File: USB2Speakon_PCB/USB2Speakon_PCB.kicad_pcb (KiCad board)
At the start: 4 copper layers, 15 x 26 mm, 51 parts, among them J1 USB_C_Receptacle_USB2.0_16P, J2 Conn_01x04, U1 PCM2912A, U2 TPA2012D2RTJR, Y1 6 MHz

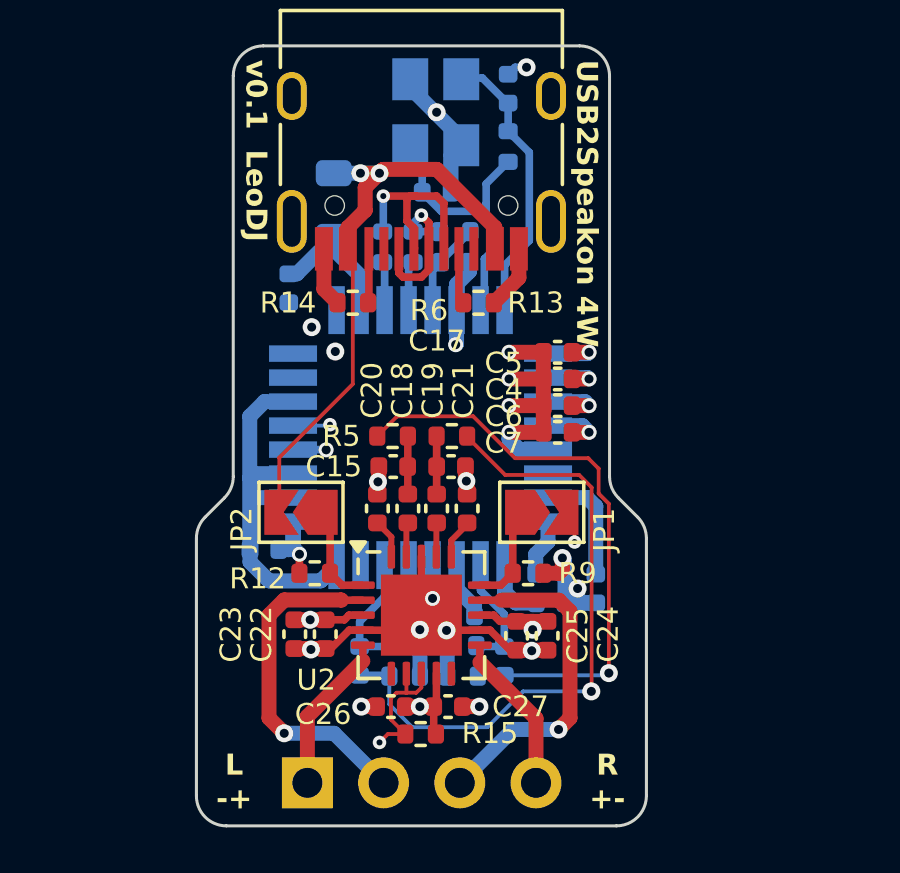
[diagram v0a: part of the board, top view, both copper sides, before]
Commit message: some minor changes, idk
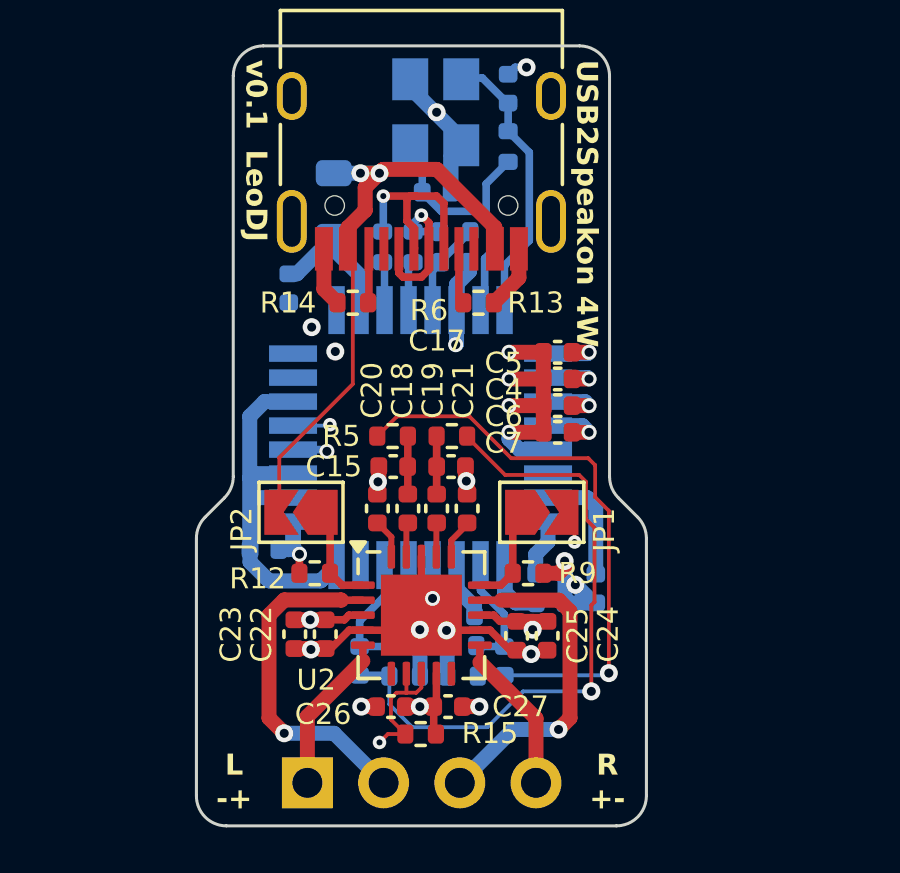
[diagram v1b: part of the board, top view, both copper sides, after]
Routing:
- net GND: track 51.2 -> 49.9 mm
